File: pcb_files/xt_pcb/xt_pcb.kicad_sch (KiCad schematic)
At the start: 31 parts, among them J1 Conn_01x04_Socket, J2 Conn_01x05, U1 XC6206PxxxMR, U2 RP2040, U3 W25Q128JVS, Y1 Crystal_GND24

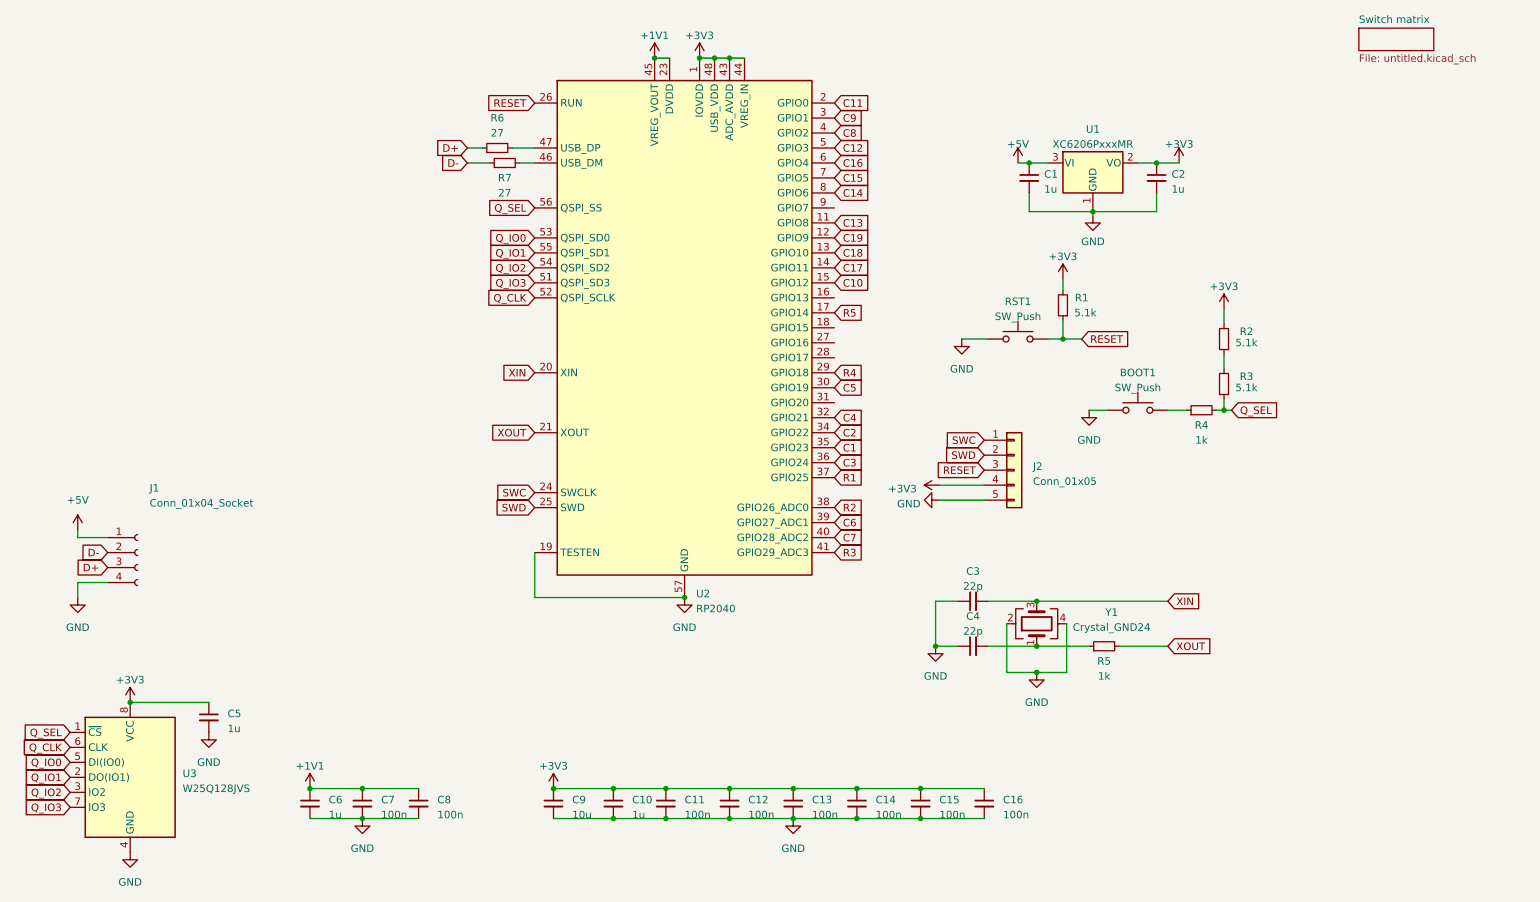
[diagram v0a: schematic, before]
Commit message: feat: new stm32 based board in progress
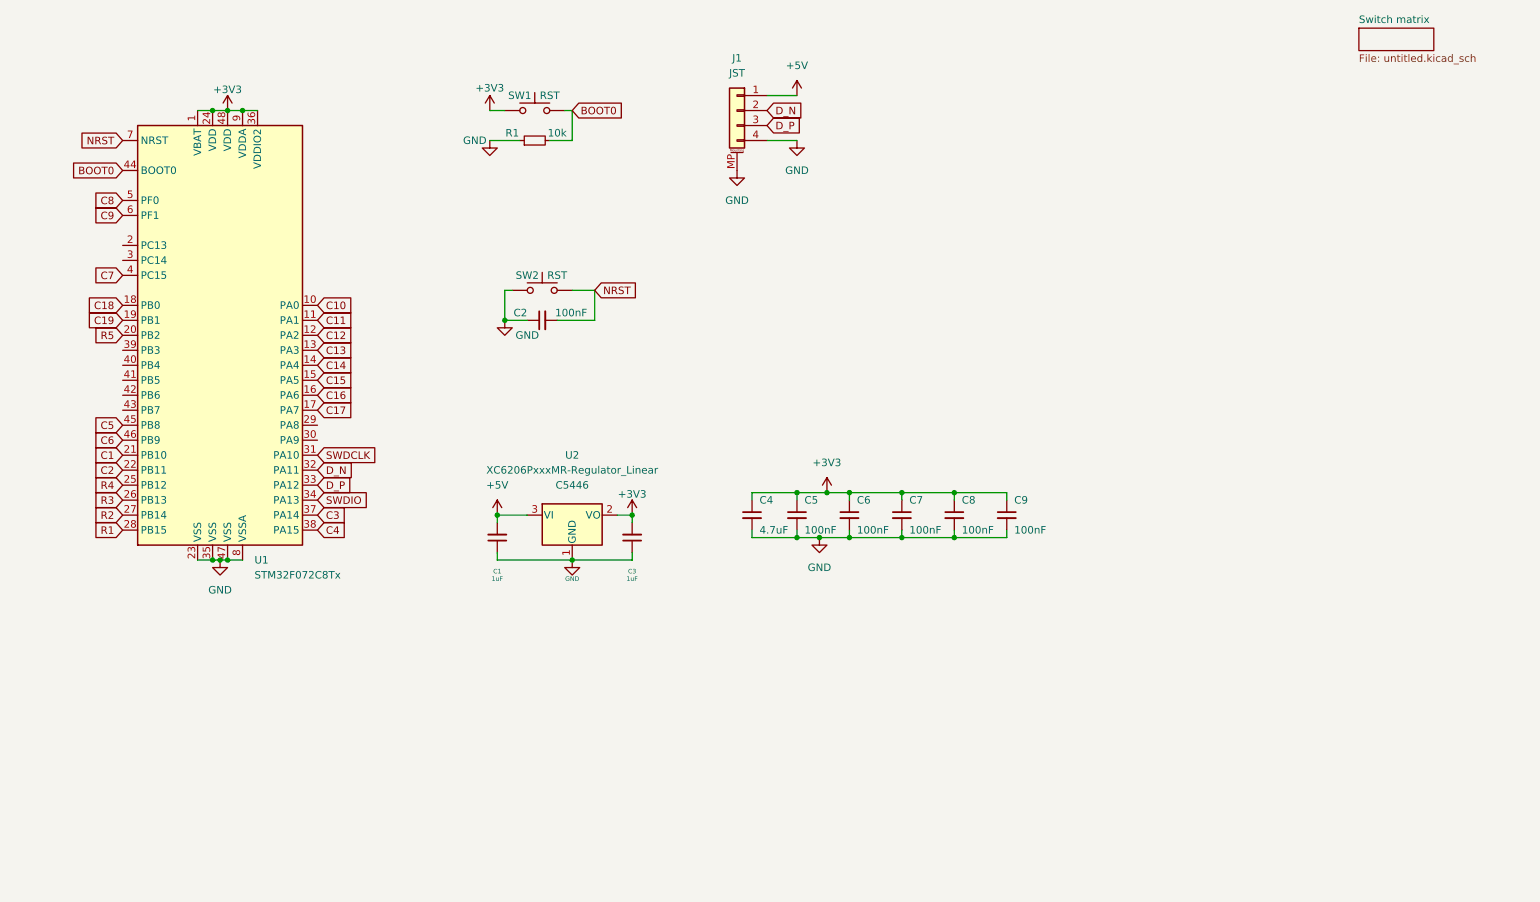
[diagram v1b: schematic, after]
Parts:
- removed BOOT1, RST1: SW_Push, Button_Switch_SMD:SW_SPST_TL3342, symbol Switch:SW_Push
- removed C10: 1u, Capacitor_SMD:C_0402_1005Metric, symbol Device:C_Small
- removed C11, C12, C13, C14, C15, C16: 100n, Capacitor_SMD:C_0402_1005Metric, symbol Device:C_Small
- removed J1: Conn_01x04_Socket, Connector_Molex:Molex_Pico-EZmate_78171-0004_1x04-1MP_P1.20mm_Vertical, symbol Connector:Conn_01x04_Socket
- removed J2: Conn_01x05, Connector_PinHeader_2.54mm:PinHeader_1x05_P2.54mm_Vertical, symbol Connector_Generic:Conn_01x05
- removed R2, R3: 5.1k, Resistor_SMD:R_0402_1005Metric, symbol Device:R_Small
- removed R4, R5: 1k, Resistor_SMD:R_0402_1005Metric, symbol Device:R_Small
- removed R6, R7: 27, Resistor_SMD:R_0402_1005Metric, symbol Device:R_Small
- removed U1: XC6206PxxxMR, Package_TO_SOT_SMD:SOT-23-3, symbol Regulator_Linear:XC6206PxxxMR
- removed U2: RP2040, Package_DFN_QFN:QFN-56-1EP_7x7mm_P0.4mm_EP3.2x3.2mm, symbol MCU_RaspberryPi:RP2040
- removed U3: W25Q128JVS, Package_SO:SOIC-8_5.23x5.23mm_P1.27mm, symbol Memory_Flash:W25Q128JVS
- removed Y1: Crystal_GND24, Crystal:Crystal_SMD_3225-4Pin_3.2x2.5mm, symbol Device:Crystal_GND24
- added J1: JST, Connector_Molex:Molex_Pico-EZmate_78171-0004_1x04-1MP_P1.20mm_Vertical, symbol Connector_Generic_MountingPin:Conn_01x04_MountingPin
- added SW1, SW2: RST, Button_Switch_SMD:SW_SPST_SKQG_WithoutStem, symbol Switch:SW_Push
- added U1: STM32F072C8Tx, Package_QFP:LQFP-48_7x7mm_P0.5mm, symbol MCU_ST_STM32F0:STM32F072C8Tx
- added U2: XC6206PxxxMR-Regulator_Linear, Package_TO_SOT_SMD:SOT-23, symbol kicad-keyboard-parts:XC6206PxxxMR-Regulator_Linear
- C1: value 1u -> 1uF; LCSC (none) -> C52923
- C2, C5, C6: value 1u -> 100nF; LCSC (none) -> C307331
- C3: value 22p -> 1uF; LCSC (none) -> C52923
- C4: value 22p -> 4.7uF; LCSC (none) -> C52923
- C7, C8: value 100n -> 100nF; LCSC (none) -> C307331
- C9: value 10u -> 100nF; footprint Capacitor_SMD:C_0603_1608Metric -> Capacitor_SMD:C_0402_1005Metric; LCSC (none) -> C307331
- R1: value 5.1k -> 10k
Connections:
- net +1V1 is gone; now on net +3V3: C6.1, C7.1, C8.1
- net RESET is gone; now on net GND: R1.1
- net XIN is gone; now on net +3V3: C3.2
- net +3V3: now also C4.1, SW1.1, U1.1 (VBAT), U1.24 (VDD), U1.36 (VDDIO2), U1.48 (VDD), U1.9 (VDDA), U2.2 (VO); no longer C2.1, R1.2
- net +5V: now also C1.2, J1.1 (Pin_1), U2.3 (VI); no longer C1.1
- net C1: now also U1.21 (PB10)
- net C10: now also U1.10 (PA0)
- net C11: now also U1.11 (PA1)
- net C12: now also U1.12 (PA2)
- net C13: now also U1.13 (PA3)
- net C14: now also U1.14 (PA4)
- net C15: now also U1.15 (PA5)
- net C16: now also U1.16 (PA6)
- net C17: now also U1.17 (PA7)
- net C18: now also U1.18 (PB0)
- net C19: now also U1.19 (PB1)
- net C2: now also U1.22 (PB11)
- net C3: now also U1.37 (PA14)
- net C4: now also U1.38 (PA15)
- net C5: now also U1.45 (PB8)
- net C6: now also U1.46 (PB9)
- net C7: now also U1.4 (PC15)
- net C8: now also U1.5 (PF0)
- net C9: now also U1.6 (PF1)
- net GND: now also C1.1, C2.1, C4.2, J1.4 (Pin_4), J1.MP (MountPin), SW2.1, U1.23 (VSS), U1.35 (VSS), U1.47 (VSS), U1.8 (VSSA), U2.1 (GND); no longer C1.2, C2.2, C4.1
- net R1: now also U1.28 (PB15)
- net R2: now also U1.27 (PB14)
- net R3: now also U1.26 (PB13)
- net R4: now also U1.25 (PB12)
- net R5: now also U1.20 (PB2)
- new net BOOT0: R1.2, SW1.2, U1.44 (BOOT0)
- new net D_N: J1.2 (Pin_2), U1.32 (PA11)
- new net D_P: J1.3 (Pin_3), U1.33 (PA12)
- new net NRST: C2.2, SW2.2, U1.7 (NRST)
- new net SWDCLK: U1.31 (PA10)
- new net SWDIO: U1.34 (PA13)
